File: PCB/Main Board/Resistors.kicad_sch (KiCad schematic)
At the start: 17 parts, among them K501 AGQ200A12, K502 AGQ200A12, K503 AGQ200A12, K504 AGQ200A12, K505 AGQ200A12

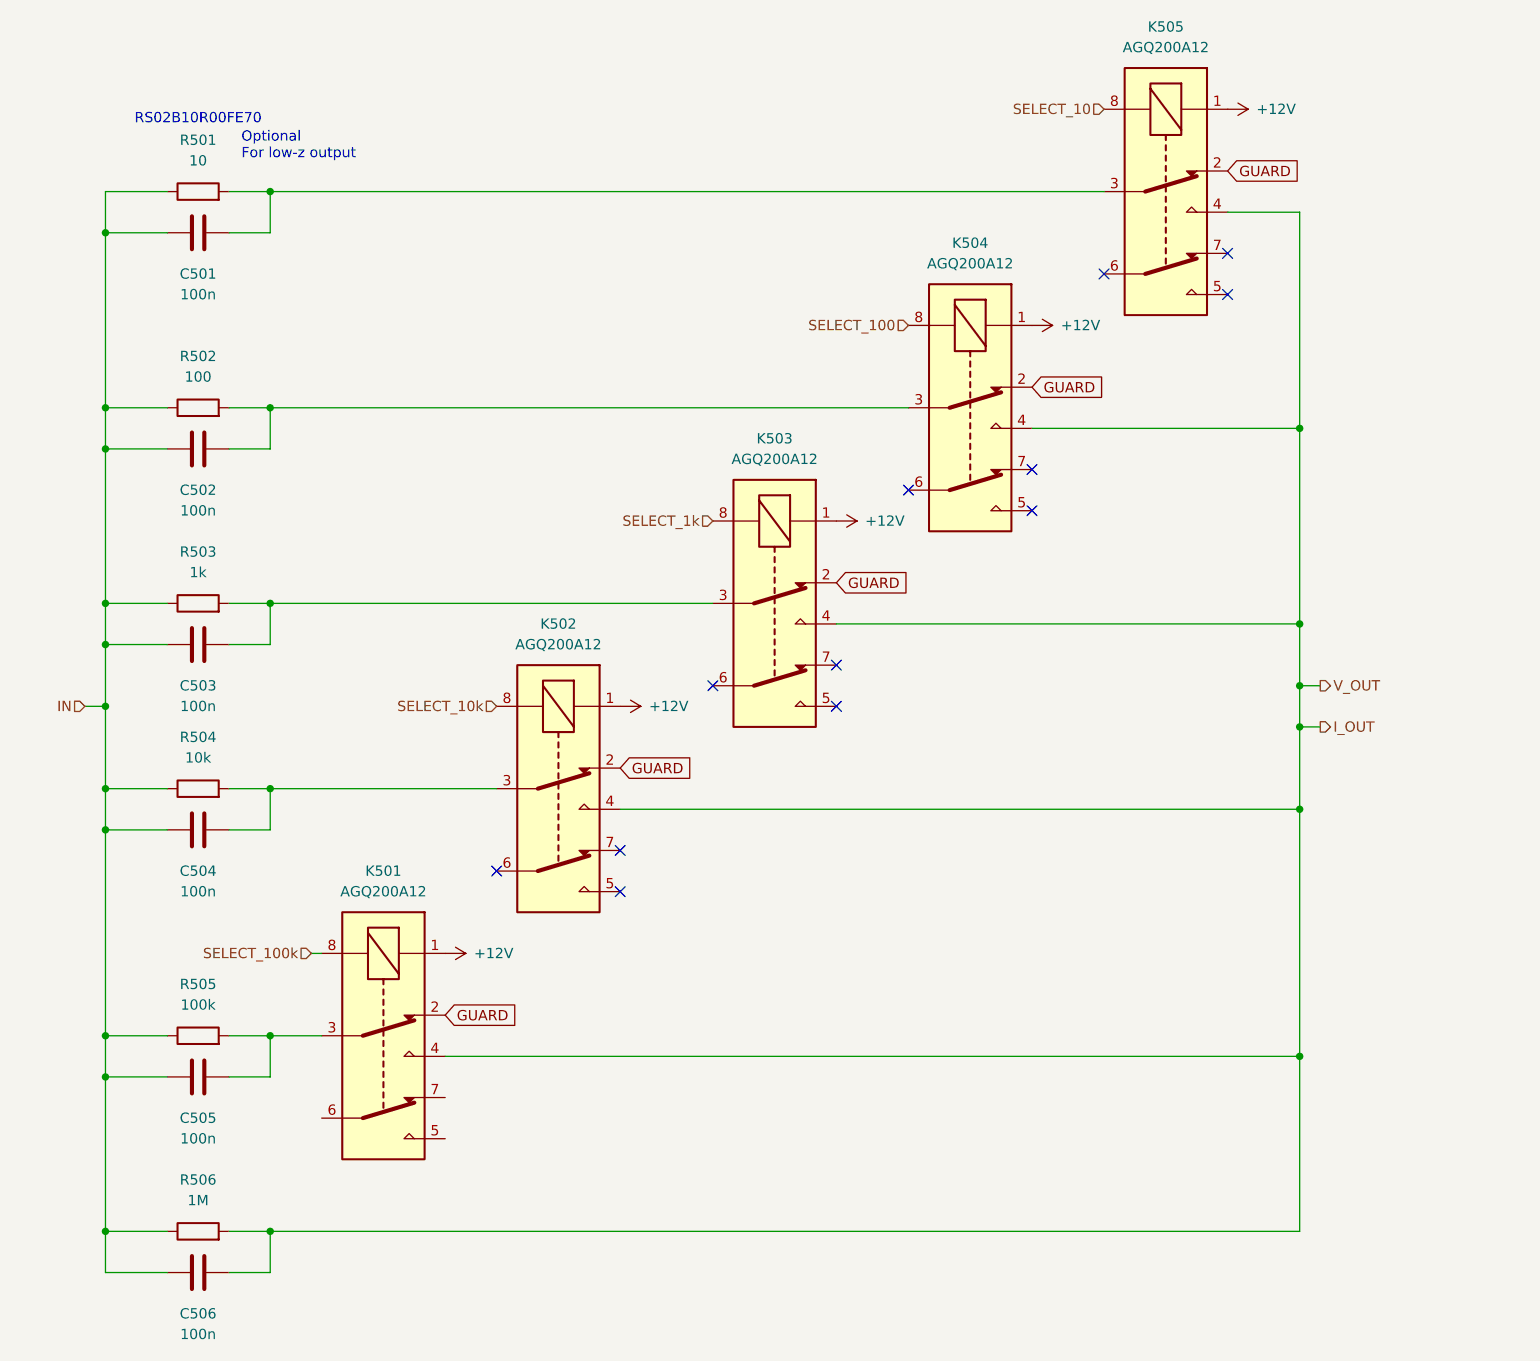
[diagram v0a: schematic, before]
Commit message: fb capacitances for abb
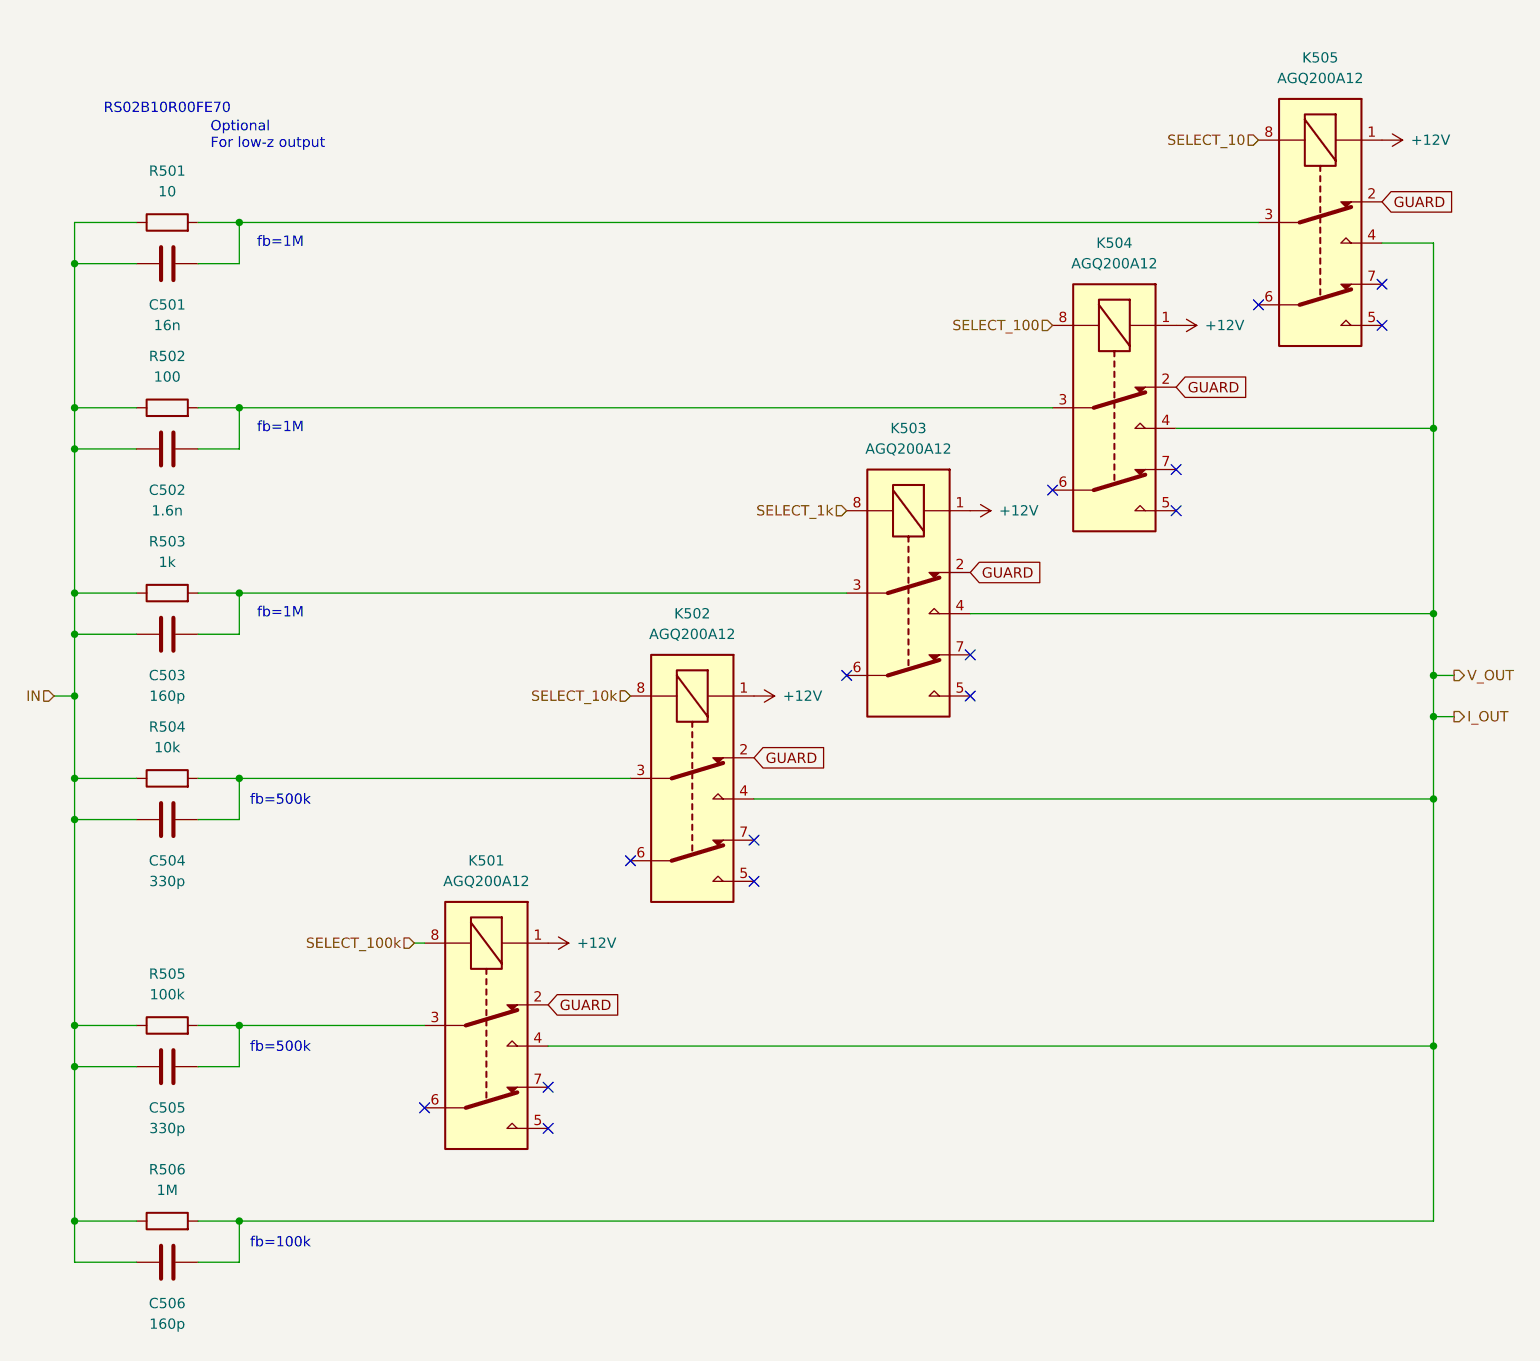
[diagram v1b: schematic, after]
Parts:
- C501: value 100n -> 16n
- C502: value 100n -> 1.6n
- C503, C506: value 100n -> 160p
- C504, C505: value 100n -> 330p
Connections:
- no-connect marks 12 -> 15
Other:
- note added: "fb=100k"
- note added: "fb=1M"
- note added: "fb=500k"
- moved on the sheet: C501, C502, C503, C504, C505, C506, K501, K502, K503, K504, K505, R501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
